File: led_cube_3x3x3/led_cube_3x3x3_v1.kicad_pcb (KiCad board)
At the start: 2 copper layers, 54 x 54 mm, 62 parts, among them IC1 ATMEGA8A-P, J1 Supply, J2 ISP, J4 UART, Q1 A1015, Q2 A1015, Q3 A1015, Q4 SFH320, U1 ST2221C, U2 24C512, X1 16MHz

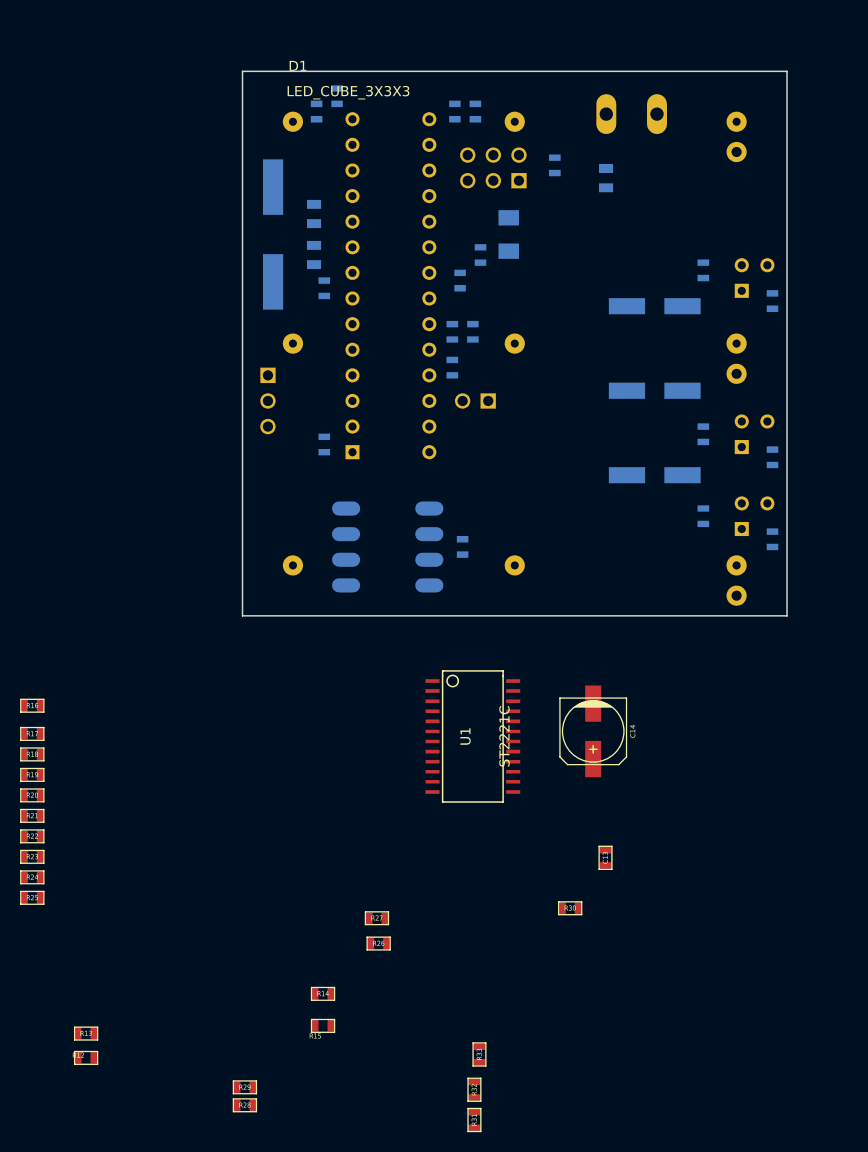
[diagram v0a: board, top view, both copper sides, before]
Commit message: led cube pcb v1.0
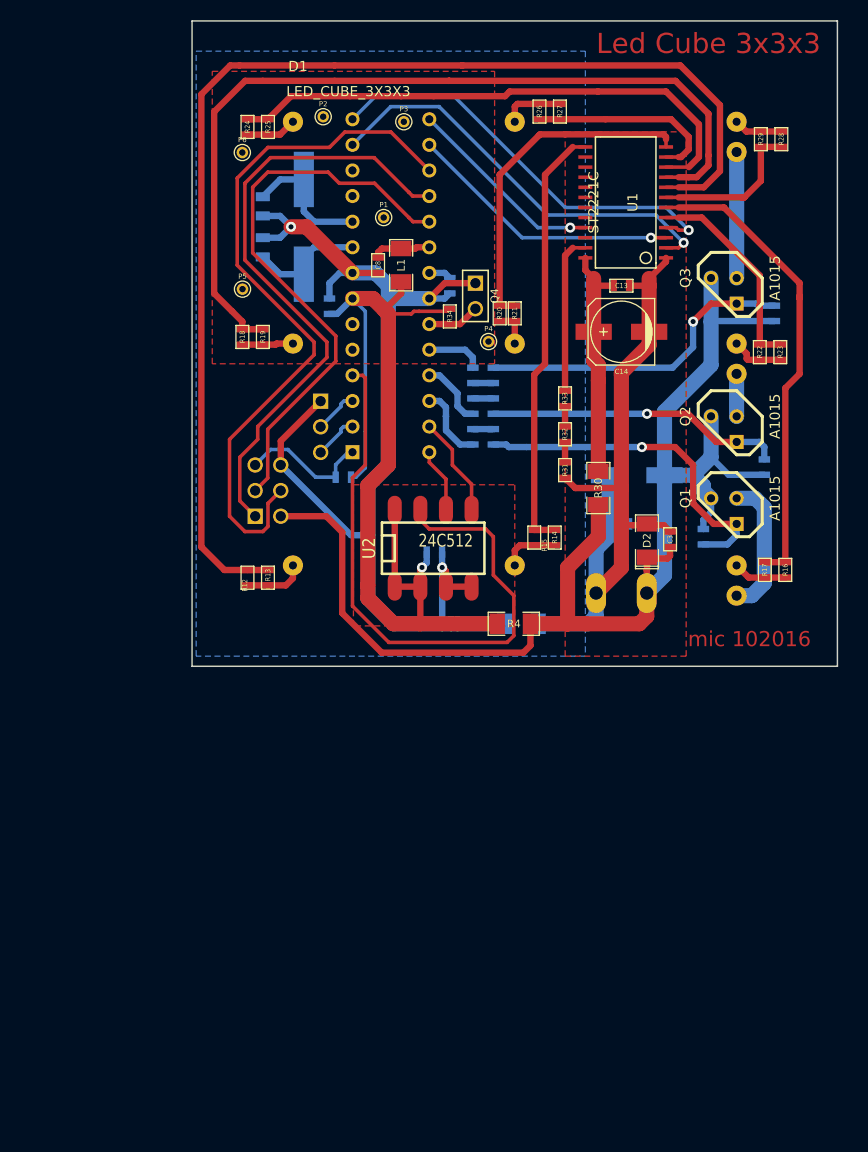
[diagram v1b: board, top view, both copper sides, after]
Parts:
- removed C4, C6: 10u, c_elec_6.3x5.3
- removed C5: 100n, SM0603
- added D2: 5v1, SM1206POL2, F.Cu at (293.1, 73.5)
- added P1: CONN_1, PINTST, F.Cu at (267.0, 41.5)
- added P2: CONN_1, PINTST, F.Cu at (261.0, 31.5)
- added P3: CONN_1, PINTST, F.Cu at (269.0, 32.0)
- added P4: CONN_1, PINTST, F.Cu at (277.4, 53.8)
- added P5: CONN_1, PINTST, F.Cu at (253.0, 48.6)
- added P6: CONN_1, PINTST, F.Cu at (253.0, 35.1)
- C3, C8, L1, Q1, Q2, Q3, Q4, R34, U2: moved to F.Cu
- R30: footprint SM0603 -> SM1206
- R35: footprint SM0805 -> SM1206
- R4: footprint SM0603 -> SM1206; moved to F.Cu
- moved R28 109.6 mm to (306.4, 33.7), turned to 90 degrees
- moved R29 107.1 mm to (304.4, 33.7), turned to 90 degrees
- moved R23 89.5 mm to (306.3, 54.8), turned to 270 degrees
- moved R22 86.7 mm to (304.3, 54.8), turned to 270 degrees
- moved R26 84.0 mm to (282.4, 31.0), turned to 90 degrees
- moved R27 82.0 mm to (284.5, 31.0), turned to 90 degrees
- moved R25 79.9 mm to (255.5, 32.5), turned to 270 degrees
- moved R24 77.4 mm to (253.5, 32.5), turned to 270 degrees
- moved R16 75.9 mm to (306.8, 76.4), turned to 270 degrees
- moved R17 74.4 mm to (304.8, 76.4), turned to 270 degrees
- moved R21 69.1 mm to (280.0, 51.0), turned to 270 degrees
- moved R20 66.6 mm to (278.5, 51.0), turned to 270 degrees
- moved R32 65.6 mm to (285.0, 63.0)
- moved R33 65.6 mm to (285.0, 59.4)
- moved R31 65.1 mm to (285.0, 66.5)
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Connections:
- C12 pad 1: +5V -> /uCVcc
- IC1 pad 11: SDI -> (no net)
- IC1 pad 12: LA -> (no net)
- IC1 pad 13: OE -> SDI
- IC1 pad 14: Lev_1 -> LA
- IC1 pad 15: Lev_2 -> OE
- IC1 pad 16: (no net) -> CLK
- IC1 pad 23: Lev_3 -> LIGHT_SENS
- IC1 pad 24: (no net) -> Lev_3
- IC1 pad 25: LIGHT_SENS -> Lev_2
- IC1 pad 26: (no net) -> Lev_1
- IC1 pad 6: CLK -> (no net)
- J1 pad 2: GND -> GNDPWR
- L1 pad 1: +5V -> /uCVcc
- Q1 pad 1: /A1C -> +5V
- Q1 pad 2: +5V -> /A1C
- Q2 pad 1: /A2C -> +5V
- Q2 pad 2: +5V -> /A2C
- Q3 pad 1: /A3C -> +5V
- Q3 pad 2: +5V -> /A3C
- R35 pad 1: GND -> GNDPWR
- R35 pad 2: GNDPWR -> GND
- U1 pad 10: Vert_6 -> Vert_7
- U1 pad 11: Vert_7 -> Vert_8
- U1 pad 12: Vert_8 -> Vert_5
- U1 pad 13: Vert_9 -> Vert_2
- U1 pad 5: Vert_1 -> Vert_6
- U1 pad 6: Vert_2 -> Vert_3
- U1 pad 7: Vert_3 -> Vert_9
- U1 pad 8: Vert_4 -> Vert_1
- U1 pad 9: Vert_5 -> Vert_4
- U2 pad 1: +5V -> /uCVcc
- U2 pad 2: +5V -> /uCVcc
- U2 pad 8: +5V -> /uCVcc
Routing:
- net +5V: track 0.00 -> 136.0 mm
- net Vert_1: track 0.00 -> 119.3 mm
- net GND: track 0.00 -> 115.0 mm, vias 0 -> 2
- net /uCVcc: track 0.00 -> 97.2 mm, vias 0 -> 1
- net Vert_4: track 0.00 -> 86.3 mm
- net GNDPWR: track 0.00 -> 72.5 mm
- net ISP MOSI: track 0.00 -> 71.4 mm
- net WP: track 0.00 -> 61.9 mm
- net ISP MISO: track 0.00 -> 61.5 mm
- net ISP SCK: track 0.00 -> 57.0 mm
- net Vert_7: track 0.00 -> 54.2 mm
- net Vert_3: track 0.00 -> 46.9 mm
- net Vert_2: track 0.00 -> 42.8 mm
- net LA: track 0.00 -> 42.1 mm, vias 0 -> 1
- net SDI: track 0.00 -> 42.0 mm, vias 0 -> 1
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- added copper zone on B.Cu, net GND
- added copper zone on F.Cu, net GND
- added copper zone on F.Cu, net GNDPWR
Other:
- board size 54 x 54 mm -> 64 x 64 mm
- board text added: "Led Cube 3x3x3"
- board text added: "mic 102016"
